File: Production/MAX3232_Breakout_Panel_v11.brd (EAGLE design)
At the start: 116.8 x 100.1 mm, 267 parts, among them U1 MAX3232, U10 MAX3232, U11 MAX3232, U12 MAX3232, U13 MAX3232, U14 MAX3232, U15 MAX3232, U16 MAX3232, U17 MAX3232, U18 MAX3232, U19 MAX3232, U2 MAX3232, U20 MAX3232, U21 MAX3232, U22 MAX3232, U23 MAX3232, U24 MAX3232, U3 MAX3232, U4 MAX3232, U5 MAX3232, U6 MAX3232, U7 MAX3232, U8 MAX3232, U9 MAX3232

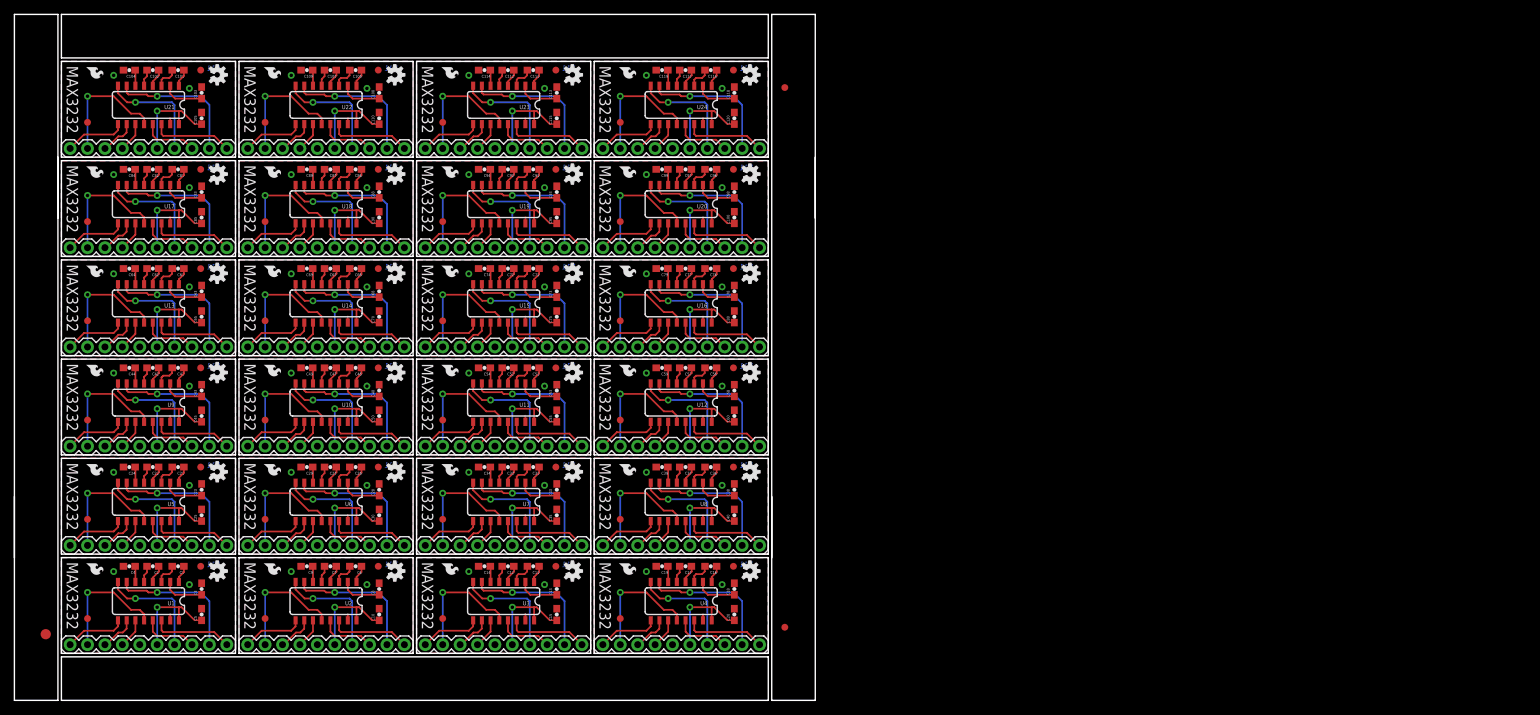
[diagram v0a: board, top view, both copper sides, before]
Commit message: New panel
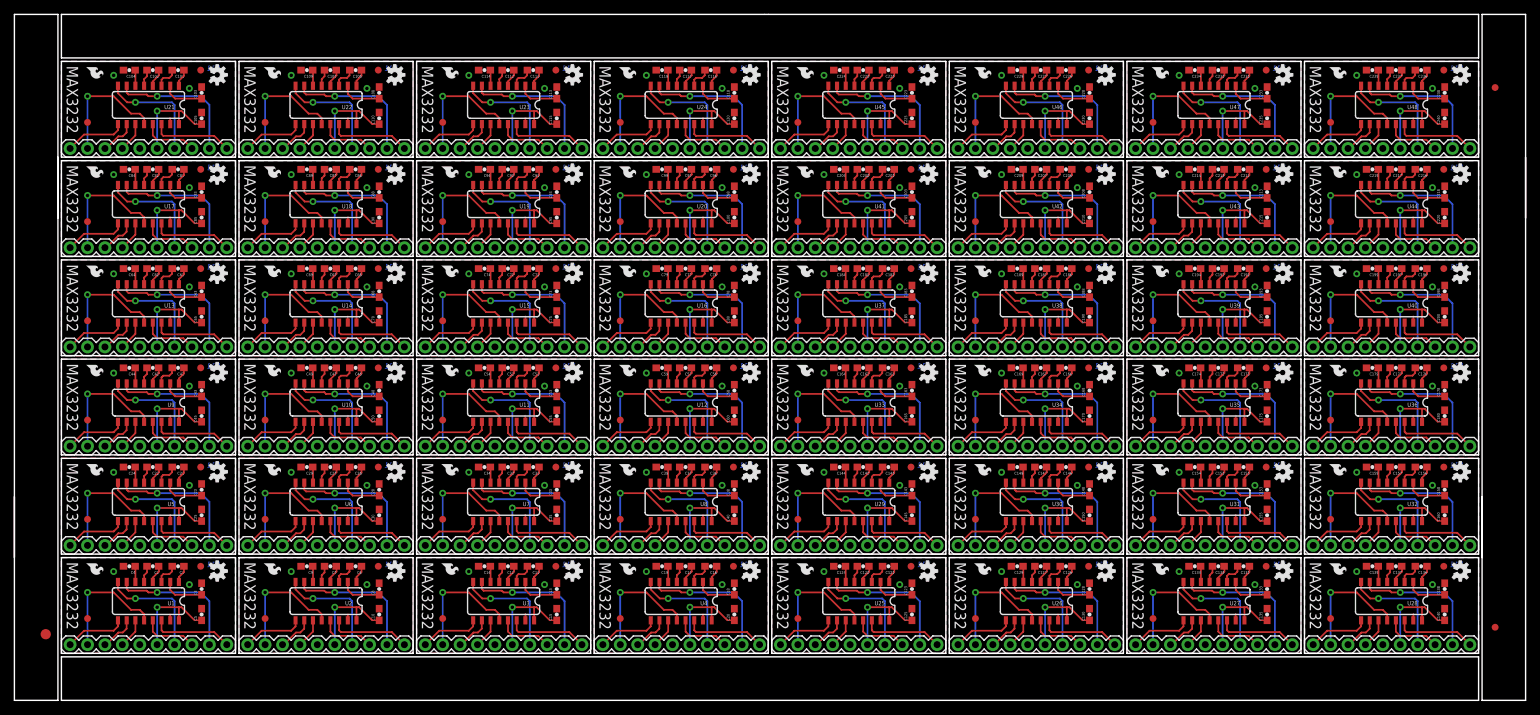
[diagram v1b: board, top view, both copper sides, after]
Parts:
- added C121, C122, C123, C124, C125, C126, C127, C128, C129, C130, C131, C132, C133, C134, C135, C136, C137, C138, C139, C140, C141, C142, C143, C144, C145, C146, C147, C148, C149, C150, C151, C152, C153, C154, C155, C156, C157, C158, C159, C160, C161, C162, C163, C164, C165, C166, C167, C168, C169, C170, C171, C172, C173, C174, C175, C176, C177, C178, C179, C180, C181, C182, C183, C184, C185, C186, C187, C188, C189, C190, C191, C192, C193, C194, C195, C196, C197, C198, C199, C200, C201, C202, C203, C204, C205, C206, C207, C208, C209, C210, C211, C212, C213, C214, C215, C216, C217, C218, C219, C220, C221, C222, C223, C224, C225, C226, C227, C228, C229, C230, C231, C232, C233, C234, C235, C236, C237, C238, C239, C240: .1uF, SparkFun-Capacitors:0603-CAP
- added FID49, FID50, FID51, FID52, FID53, FID54, FID55, FID56, FID57, FID58, FID59, FID60, FID61, FID62, FID63, FID64, FID65, FID66, FID67, FID68, FID69, FID70, FID71, FID72, FID73, FID74, FID75, FID76, FID77, FID78, FID79, FID80, FID81, FID82, FID83, FID84, FID85, FID86, FID87, FID88, FID89, FID90, FID91, FID92, FID93, FID94, FID95, FID96: FIDUCIAL1X2, SparkFun-Aesthetics:FIDUCIAL-1X2
- added JP25, JP26, JP27, JP28, JP29, JP30, JP31, JP32, JP33, JP34, JP35, JP36, JP37, JP38, JP39, JP40, JP41, JP42, JP43, JP44, JP45, JP46, JP47, JP48: M10", SparkFun-Connectors:1X10
- added LOGO25, LOGO26, LOGO27, LOGO28, LOGO29, LOGO30, LOGO31, LOGO32, LOGO33, LOGO34, LOGO35, LOGO36, LOGO37, LOGO38, LOGO39, LOGO40, LOGO41, LOGO42, LOGO43, LOGO44, LOGO45, LOGO46, LOGO47, LOGO48: SFE_LOGO_FLAME.1_INCH, SparkFun-Aesthetics:SFE_LOGO_FLAME_.1
- added U$25, U$26, U$27, U$28, U$29, U$30, U$31, U$32, U$33, U$34, U$35, U$36, U$37, U$38, U$39, U$40, U$41, U$42, U$43, U$44, U$45, U$46, U$47, U$48: OSHW-LOGOS, SparkFun-Aesthetics:OSHW-LOGO-S
- added U25, U26, U27, U28, U29, U30, U31, U32, U33, U34, U35, U36, U37, U38, U39, U40, U41, U42, U43, U44, U45, U46, U47, U48: MAX3232, SparkFun-DigitalIC:SO016
- moved E$4 103.6 mm to (216.0, 10.7)
- moved E$5 103.6 mm to (216.0, 89.4)
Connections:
- new net C1+24: C121.1, U25.1
- new net C1+25: C126.1, U26.1
- new net C1+26: C131.1, U27.1
- new net C1+27: C136.1, U28.1
- new net C1+28: C141.1, U29.1
- new net C1+29: C146.1, U30.1
- new net C1+30: C151.1, U31.1
- new net C1+31: C156.1, U32.1
- new net C1+32: C161.1, U33.1
- new net C1+33: C166.1, U34.1
- new net C1+34: C171.1, U35.1
- new net C1+35: C176.1, U36.1
- new net C1+36: C181.1, U37.1
- new net C1+37: C186.1, U38.1
- new net C1+38: C191.1, U39.1
- new net C1+39: C196.1, U40.1
- new net C1+40: C201.1, U41.1
- new net C1+41: C206.1, U42.1
- new net C1+42: C211.1, U43.1
- new net C1+43: C216.1, U44.1
- new net C1+44: C221.1, U45.1
- new net C1+45: C226.1, U46.1
- new net C1+46: C231.1, U47.1
- new net C1+47: C236.1, U48.1
- new net C1-24: C121.2, U25.3
- new net C1-25: C126.2, U26.3
- new net C1-26: C131.2, U27.3
- new net C1-27: C136.2, U28.3
- new net C1-28: C141.2, U29.3
- new net C1-29: C146.2, U30.3
- new net C1-30: C151.2, U31.3
- new net C1-31: C156.2, U32.3
- new net C1-32: C161.2, U33.3
- new net C1-33: C166.2, U34.3
- new net C1-34: C171.2, U35.3
- new net C1-35: C176.2, U36.3
- new net C1-36: C181.2, U37.3
- new net C1-37: C186.2, U38.3
- new net C1-38: C191.2, U39.3
- new net C1-39: C196.2, U40.3
- new net C1-40: C201.2, U41.3
- new net C1-41: C206.2, U42.3
- new net C1-42: C211.2, U43.3
- new net C1-43: C216.2, U44.3
- new net C1-44: C221.2, U45.3
- new net C1-45: C226.2, U46.3
- new net C1-46: C231.2, U47.3
- new net C1-47: C236.2, U48.3
- new net C2+24: C122.1, U25.4
- new net C2+25: C127.1, U26.4
- new net C2+26: C132.1, U27.4
- new net C2+27: C137.1, U28.4
- new net C2+28: C142.1, U29.4
- new net C2+29: C147.1, U30.4
- new net C2+30: C152.1, U31.4
- new net C2+31: C157.1, U32.4
- new net C2+32: C162.1, U33.4
- new net C2+33: C167.1, U34.4
- new net C2+34: C172.1, U35.4
- new net C2+35: C177.1, U36.4
- new net C2+36: C182.1, U37.4
- new net C2+37: C187.1, U38.4
- new net C2+38: C192.1, U39.4
- new net C2+39: C197.1, U40.4
- new net C2+40: C202.1, U41.4
- new net C2+41: C207.1, U42.4
- new net C2+42: C212.1, U43.4
- new net C2+43: C217.1, U44.4
- new net C2+44: C222.1, U45.4
- new net C2+45: C227.1, U46.4
- new net C2+46: C232.1, U47.4
- new net C2+47: C237.1, U48.4
- new net C2-24: C122.2, U25.5
- new net C2-25: C127.2, U26.5
- new net C2-26: C132.2, U27.5
- new net C2-27: C137.2, U28.5
- new net C2-28: C142.2, U29.5
- new net C2-29: C147.2, U30.5
- new net C2-30: C152.2, U31.5
- new net C2-31: C157.2, U32.5
- new net C2-32: C162.2, U33.5
- new net C2-33: C167.2, U34.5
- new net C2-34: C172.2, U35.5
- new net C2-35: C177.2, U36.5
- new net C2-36: C182.2, U37.5
- new net C2-37: C187.2, U38.5
- new net C2-38: C192.2, U39.5
- new net C2-39: C197.2, U40.5
- new net C2-40: C202.2, U41.5
- new net C2-41: C207.2, U42.5
- new net C2-42: C212.2, U43.5
- new net C2-43: C217.2, U44.5
- new net C2-44: C222.2, U45.5
- new net C2-45: C227.2, U46.5
- new net C2-46: C232.2, U47.5
- new net C2-47: C237.2, U48.5
- new net GND24: C123.2, C124.2, C125.2, JP25.6, U25.15
- new net GND25: C128.2, C129.2, C130.2, JP26.6, U26.15
- new net GND26: C133.2, C134.2, C135.2, JP27.6, U27.15
- new net GND27: C138.2, C139.2, C140.2, JP28.6, U28.15
- new net GND28: C143.2, C144.2, C145.2, JP29.6, U29.15
- new net GND29: C148.2, C149.2, C150.2, JP30.6, U30.15
- new net GND30: C153.2, C154.2, C155.2, JP31.6, U31.15
- new net GND31: C158.2, C159.2, C160.2, JP32.6, U32.15
- new net GND32: C163.2, C164.2, C165.2, JP33.6, U33.15
- new net GND33: C168.2, C169.2, C170.2, JP34.6, U34.15
- new net GND34: C173.2, C174.2, C175.2, JP35.6, U35.15
- new net GND35: C178.2, C179.2, C180.2, JP36.6, U36.15
- new net GND36: C183.2, C184.2, C185.2, JP37.6, U37.15
- new net GND37: C188.2, C189.2, C190.2, JP38.6, U38.15
- new net GND38: C193.2, C194.2, C195.2, JP39.6, U39.15
- new net GND39: C198.2, C199.2, C200.2, JP40.6, U40.15
- new net GND40: C203.2, C204.2, C205.2, JP41.6, U41.15
- new net GND41: C208.2, C209.2, C210.2, JP42.6, U42.15
- new net GND42: C213.2, C214.2, C215.2, JP43.6, U43.15
- new net GND43: C218.2, C219.2, C220.2, JP44.6, U44.15
- new net GND44: C223.2, C224.2, C225.2, JP45.6, U45.15
- new net GND45: C228.2, C229.2, C230.2, JP46.6, U46.15
- new net GND46: C233.2, C234.2, C235.2, JP47.6, U47.15
- new net GND47: C238.2, C239.2, C240.2, JP48.6, U48.15
- new net R1IN24: JP25.3, U25.13
- new net R1IN25: JP26.3, U26.13
- new net R1IN26: JP27.3, U27.13
- new net R1IN27: JP28.3, U28.13
- new net R1IN28: JP29.3, U29.13
- new net R1IN29: JP30.3, U30.13
- new net R1IN30: JP31.3, U31.13
- new net R1IN31: JP32.3, U32.13
- new net R1IN32: JP33.3, U33.13
- new net R1IN33: JP34.3, U34.13
- new net R1IN34: JP35.3, U35.13
- new net R1IN35: JP36.3, U36.13
- new net R1IN36: JP37.3, U37.13
- new net R1IN37: JP38.3, U38.13
- new net R1IN38: JP39.3, U39.13
- new net R1IN39: JP40.3, U40.13
- new net R1IN40: JP41.3, U41.13
- new net R1IN41: JP42.3, U42.13
- new net R1IN42: JP43.3, U43.13
- new net R1IN43: JP44.3, U44.13
- new net R1IN44: JP45.3, U45.13
- new net R1IN45: JP46.3, U46.13
- new net R1IN46: JP47.3, U47.13
- new net R1IN47: JP48.3, U48.13
- new net R1OUT24: JP25.9, U25.12
- new net R1OUT25: JP26.9, U26.12
- new net R1OUT26: JP27.9, U27.12
- new net R1OUT27: JP28.9, U28.12
- new net R1OUT28: JP29.9, U29.12
- new net R1OUT29: JP30.9, U30.12
- new net R1OUT30: JP31.9, U31.12
- new net R1OUT31: JP32.9, U32.12
- new net R1OUT32: JP33.9, U33.12
- new net R1OUT33: JP34.9, U34.12
- new net R1OUT34: JP35.9, U35.12
- new net R1OUT35: JP36.9, U36.12
- new net R1OUT36: JP37.9, U37.12
- new net R1OUT37: JP38.9, U38.12
- new net R1OUT38: JP39.9, U39.12
- new net R1OUT39: JP40.9, U40.12
- new net R1OUT40: JP41.9, U41.12
- new net R1OUT41: JP42.9, U42.12
- new net R1OUT42: JP43.9, U43.12
- new net R1OUT43: JP44.9, U44.12
- new net R1OUT44: JP45.9, U45.12
- new net R1OUT45: JP46.9, U46.12
- new net R1OUT46: JP47.9, U47.12
- new net R1OUT47: JP48.9, U48.12
- new net R2IN24: JP25.4, U25.8
- new net R2IN25: JP26.4, U26.8
- new net R2IN26: JP27.4, U27.8
- new net R2IN27: JP28.4, U28.8
- new net R2IN28: JP29.4, U29.8
- new net R2IN29: JP30.4, U30.8
- new net R2IN30: JP31.4, U31.8
- new net R2IN31: JP32.4, U32.8
- new net R2IN32: JP33.4, U33.8
- new net R2IN33: JP34.4, U34.8
- new net R2IN34: JP35.4, U35.8
- new net R2IN35: JP36.4, U36.8
- new net R2IN36: JP37.4, U37.8
- new net R2IN37: JP38.4, U38.8
- new net R2IN38: JP39.4, U39.8
- new net R2IN39: JP40.4, U40.8
- new net R2IN40: JP41.4, U41.8
- new net R2IN41: JP42.4, U42.8
- new net R2IN42: JP43.4, U43.8
- new net R2IN43: JP44.4, U44.8
- new net R2IN44: JP45.4, U45.8
- new net R2IN45: JP46.4, U46.8
- new net R2IN46: JP47.4, U47.8
- new net R2IN47: JP48.4, U48.8
- new net R2OUT24: JP25.10, U25.9
- new net R2OUT25: JP26.10, U26.9
- new net R2OUT26: JP27.10, U27.9
- new net R2OUT27: JP28.10, U28.9
- new net R2OUT28: JP29.10, U29.9
- new net R2OUT29: JP30.10, U30.9
- new net R2OUT30: JP31.10, U31.9
- new net R2OUT31: JP32.10, U32.9
- new net R2OUT32: JP33.10, U33.9
- new net R2OUT33: JP34.10, U34.9
- new net R2OUT34: JP35.10, U35.9
- new net R2OUT35: JP36.10, U36.9
- new net R2OUT36: JP37.10, U37.9
- new net R2OUT37: JP38.10, U38.9
- new net R2OUT38: JP39.10, U39.9
- new net R2OUT39: JP40.10, U40.9
- new net R2OUT40: JP41.10, U41.9
- new net R2OUT41: JP42.10, U42.9
- new net R2OUT42: JP43.10, U43.9
- new net R2OUT43: JP44.10, U44.9
- new net R2OUT44: JP45.10, U45.9
- new net R2OUT45: JP46.10, U46.9
- new net R2OUT46: JP47.10, U47.9
- new net R2OUT47: JP48.10, U48.9
- new net T1IN24: JP25.7, U25.11
- new net T1IN25: JP26.7, U26.11
- new net T1IN26: JP27.7, U27.11
- new net T1IN27: JP28.7, U28.11
- new net T1IN28: JP29.7, U29.11
- new net T1IN29: JP30.7, U30.11
- new net T1IN30: JP31.7, U31.11
- new net T1IN31: JP32.7, U32.11
- new net T1IN32: JP33.7, U33.11
- new net T1IN33: JP34.7, U34.11
- new net T1IN34: JP35.7, U35.11
- new net T1IN35: JP36.7, U36.11
- new net T1IN36: JP37.7, U37.11
- new net T1IN37: JP38.7, U38.11
- new net T1IN38: JP39.7, U39.11
- new net T1IN39: JP40.7, U40.11
- new net T1IN40: JP41.7, U41.11
- new net T1IN41: JP42.7, U42.11
- new net T1IN42: JP43.7, U43.11
- new net T1IN43: JP44.7, U44.11
- new net T1IN44: JP45.7, U45.11
- new net T1IN45: JP46.7, U46.11
- new net T1IN46: JP47.7, U47.11
- new net T1IN47: JP48.7, U48.11
- new net T1OUT24: JP25.1, U25.14
- new net T1OUT25: JP26.1, U26.14
- new net T1OUT26: JP27.1, U27.14
- new net T1OUT27: JP28.1, U28.14
- new net T1OUT28: JP29.1, U29.14
- new net T1OUT29: JP30.1, U30.14
- new net T1OUT30: JP31.1, U31.14
- new net T1OUT31: JP32.1, U32.14
- new net T1OUT32: JP33.1, U33.14
- new net T1OUT33: JP34.1, U34.14
- new net T1OUT34: JP35.1, U35.14
- new net T1OUT35: JP36.1, U36.14
- new net T1OUT36: JP37.1, U37.14
- new net T1OUT37: JP38.1, U38.14
- new net T1OUT38: JP39.1, U39.14
- new net T1OUT39: JP40.1, U40.14
- new net T1OUT40: JP41.1, U41.14
- new net T1OUT41: JP42.1, U42.14
- new net T1OUT42: JP43.1, U43.14
- new net T1OUT43: JP44.1, U44.14
- new net T1OUT44: JP45.1, U45.14
- new net T1OUT45: JP46.1, U46.14
- new net T1OUT46: JP47.1, U47.14
- new net T1OUT47: JP48.1, U48.14
- new net T2IN24: JP25.8, U25.10
- new net T2IN25: JP26.8, U26.10
- new net T2IN26: JP27.8, U27.10
- new net T2IN27: JP28.8, U28.10
- new net T2IN28: JP29.8, U29.10
- new net T2IN29: JP30.8, U30.10
- new net T2IN30: JP31.8, U31.10
- new net T2IN31: JP32.8, U32.10
- new net T2IN32: JP33.8, U33.10
- new net T2IN33: JP34.8, U34.10
- new net T2IN34: JP35.8, U35.10
- new net T2IN35: JP36.8, U36.10
- new net T2IN36: JP37.8, U37.10
- new net T2IN37: JP38.8, U38.10
- new net T2IN38: JP39.8, U39.10
- new net T2IN39: JP40.8, U40.10
- new net T2IN40: JP41.8, U41.10
- new net T2IN41: JP42.8, U42.10
- new net T2IN42: JP43.8, U43.10
- new net T2IN43: JP44.8, U44.10
- new net T2IN44: JP45.8, U45.10
- new net T2IN45: JP46.8, U46.10
- new net T2IN46: JP47.8, U47.10
- new net T2IN47: JP48.8, U48.10
- new net T2OUT24: JP25.2, U25.7
- new net T2OUT25: JP26.2, U26.7
- new net T2OUT26: JP27.2, U27.7
- new net T2OUT27: JP28.2, U28.7
- new net T2OUT28: JP29.2, U29.7
- new net T2OUT29: JP30.2, U30.7
- new net T2OUT30: JP31.2, U31.7
- new net T2OUT31: JP32.2, U32.7
- new net T2OUT32: JP33.2, U33.7
- new net T2OUT33: JP34.2, U34.7
- new net T2OUT34: JP35.2, U35.7
- new net T2OUT35: JP36.2, U36.7
- new net T2OUT36: JP37.2, U37.7
- new net T2OUT37: JP38.2, U38.7
- new net T2OUT38: JP39.2, U39.7
- new net T2OUT39: JP40.2, U40.7
- new net T2OUT40: JP41.2, U41.7
- new net T2OUT41: JP42.2, U42.7
- new net T2OUT42: JP43.2, U43.7
- new net T2OUT43: JP44.2, U44.7
- new net T2OUT44: JP45.2, U45.7
- new net T2OUT45: JP46.2, U46.7
- new net T2OUT46: JP47.2, U47.7
- new net T2OUT47: JP48.2, U48.7
- new net V+24: C123.1, U25.2
- new net V+25: C128.1, U26.2
- new net V+26: C133.1, U27.2
- new net V+27: C138.1, U28.2
- new net V+28: C143.1, U29.2
- new net V+29: C148.1, U30.2
- new net V+30: C153.1, U31.2
- new net V+31: C158.1, U32.2
- new net V+32: C163.1, U33.2
- new net V+33: C168.1, U34.2
- new net V+34: C173.1, U35.2
- new net V+35: C178.1, U36.2
- new net V+36: C183.1, U37.2
- new net V+37: C188.1, U38.2
- new net V+38: C193.1, U39.2
- new net V+39: C198.1, U40.2
- new net V+40: C203.1, U41.2
- new net V+41: C208.1, U42.2
- new net V+42: C213.1, U43.2
- new net V+43: C218.1, U44.2
- new net V+44: C223.1, U45.2
- new net V+45: C228.1, U46.2
- new net V+46: C233.1, U47.2
- new net V+47: C238.1, U48.2
- new net V-24: C124.1, U25.6
- new net V-25: C129.1, U26.6
- new net V-26: C134.1, U27.6
- new net V-27: C139.1, U28.6
- new net V-28: C144.1, U29.6
- new net V-29: C149.1, U30.6
- new net V-30: C154.1, U31.6
- new net V-31: C159.1, U32.6
- new net V-32: C164.1, U33.6
- new net V-33: C169.1, U34.6
- new net V-34: C174.1, U35.6
- new net V-35: C179.1, U36.6
- new net V-36: C184.1, U37.6
- new net V-37: C189.1, U38.6
- new net V-38: C194.1, U39.6
- new net V-39: C199.1, U40.6
- new net V-40: C204.1, U41.6
- new net V-41: C209.1, U42.6
- new net V-42: C214.1, U43.6
- new net V-43: C219.1, U44.6
- new net V-44: C224.1, U45.6
- new net V-45: C229.1, U46.6
- new net V-46: C234.1, U47.6
- new net V-47: C239.1, U48.6
- new net VCC24: C125.1, JP25.5, U25.16
- new net VCC25: C130.1, JP26.5, U26.16
- new net VCC26: C135.1, JP27.5, U27.16
- new net VCC27: C140.1, JP28.5, U28.16
- new net VCC28: C145.1, JP29.5, U29.16
- new net VCC29: C150.1, JP30.5, U30.16
- new net VCC30: C155.1, JP31.5, U31.16
- new net VCC31: C160.1, JP32.5, U32.16
- new net VCC32: C165.1, JP33.5, U33.16
- new net VCC33: C170.1, JP34.5, U34.16
- new net VCC34: C175.1, JP35.5, U35.16
- new net VCC35: C180.1, JP36.5, U36.16
- new net VCC36: C185.1, JP37.5, U37.16
- new net VCC37: C190.1, JP38.5, U38.16
- new net VCC38: C195.1, JP39.5, U39.16
- new net VCC39: C200.1, JP40.5, U40.16
- new net VCC40: C205.1, JP41.5, U41.16
- new net VCC41: C210.1, JP42.5, U42.16
- new net VCC42: C215.1, JP43.5, U43.16
- new net VCC43: C220.1, JP44.5, U44.16
- new net VCC44: C225.1, JP45.5, U45.16
- new net VCC45: C230.1, JP46.5, U46.16
- new net VCC46: C235.1, JP47.5, U47.16
- new net VCC47: C240.1, JP48.5, U48.16
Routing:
- net T2OUT44: track 0.00 -> 20.2 mm, vias 0 -> 1
- net T2OUT36: track 0.00 -> 20.2 mm, vias 0 -> 1
- net T2OUT24: track 0.00 -> 20.2 mm, vias 0 -> 1
- net T2OUT32: track 0.00 -> 20.2 mm, vias 0 -> 1
- net T2OUT28: track 0.00 -> 20.2 mm, vias 0 -> 1
- net T2OUT47: track 0.00 -> 20.2 mm, vias 0 -> 1
- net T2OUT46: track 0.00 -> 20.2 mm, vias 0 -> 1
- net T2OUT39: track 0.00 -> 20.2 mm, vias 0 -> 1
- net T2OUT38: track 0.00 -> 20.2 mm, vias 0 -> 1
- net T2OUT45: track 0.00 -> 20.2 mm, vias 0 -> 1
- net T2OUT40: track 0.00 -> 20.2 mm, vias 0 -> 1
- net T2OUT37: track 0.00 -> 20.2 mm, vias 0 -> 1
- net T2OUT35: track 0.00 -> 20.2 mm, vias 0 -> 1
- net T2OUT34: track 0.00 -> 20.2 mm, vias 0 -> 1
- net T2OUT31: track 0.00 -> 20.2 mm, vias 0 -> 1
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- added copper zone on layer 1, net GND24
- added copper zone on layer 16, net GND24
- added copper zone on layer 1, net GND25
- added copper zone on layer 16, net GND25
- added copper zone on layer 1, net GND26
- added copper zone on layer 16, net GND26
- added copper zone on layer 1, net GND27
- added copper zone on layer 16, net GND27
- added copper zone on layer 1, net GND28
- added copper zone on layer 16, net GND28
- added copper zone on layer 1, net GND29
- added copper zone on layer 16, net GND29
- added copper zone on layer 1, net GND30
- added copper zone on layer 16, net GND30
- added copper zone on layer 1, net GND31
- added copper zone on layer 16, net GND31
- added copper zone on layer 1, net GND32
- added copper zone on layer 16, net GND32
- added copper zone on layer 1, net GND33
- added copper zone on layer 16, net GND33
- added copper zone on layer 1, net GND34
- added copper zone on layer 16, net GND34
- added copper zone on layer 1, net GND35
- added copper zone on layer 16, net GND35
- added copper zone on layer 1, net GND36
- added copper zone on layer 16, net GND36
- added copper zone on layer 1, net GND37
- added copper zone on layer 16, net GND37
- added copper zone on layer 1, net GND38
- added copper zone on layer 16, net GND38
- added copper zone on layer 1, net GND39
- added copper zone on layer 16, net GND39
- added copper zone on layer 1, net GND40
- added copper zone on layer 16, net GND40
- added copper zone on layer 1, net GND41
- added copper zone on layer 16, net GND41
- added copper zone on layer 1, net GND42
- added copper zone on layer 16, net GND42
- added copper zone on layer 1, net GND43
- added copper zone on layer 16, net GND43
- added copper zone on layer 1, net GND44
- added copper zone on layer 16, net GND44
- added copper zone on layer 1, net GND45
- added copper zone on layer 16, net GND45
- added copper zone on layer 1, net GND46
- added copper zone on layer 16, net GND46
- added copper zone on layer 1, net GND47
- added copper zone on layer 16, net GND47
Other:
- board size 116.8 x 100.1 mm -> 220.5 x 100.1 mm
